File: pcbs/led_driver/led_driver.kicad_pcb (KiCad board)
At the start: 2 copper layers, 21 parts, among them J1 Barrel_Jack, J2 greenLED, J3 Conn_Coaxial, J4 Conn_Coaxial, J5 UVLED, U1 RCD-24, U2 LM350_TO220_9V_output, U3 RCD-24

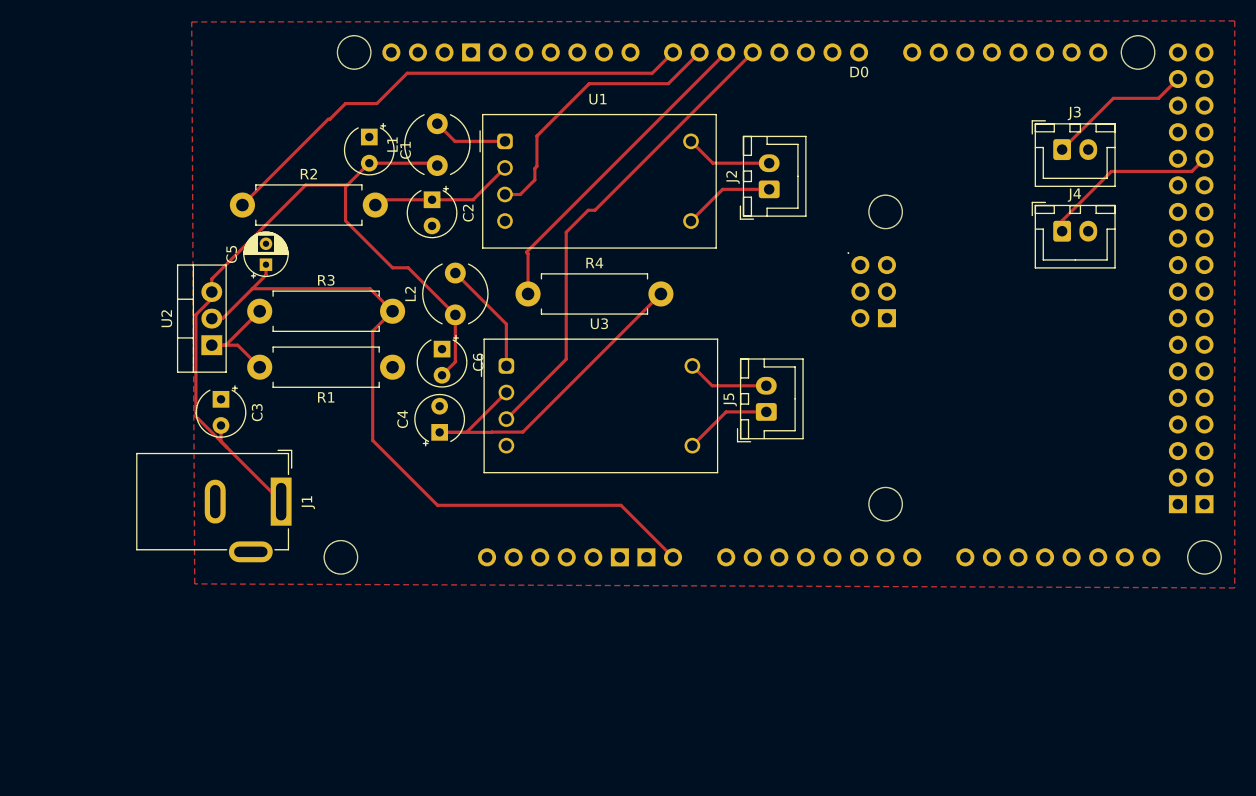
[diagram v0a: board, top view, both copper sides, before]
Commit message: update led der
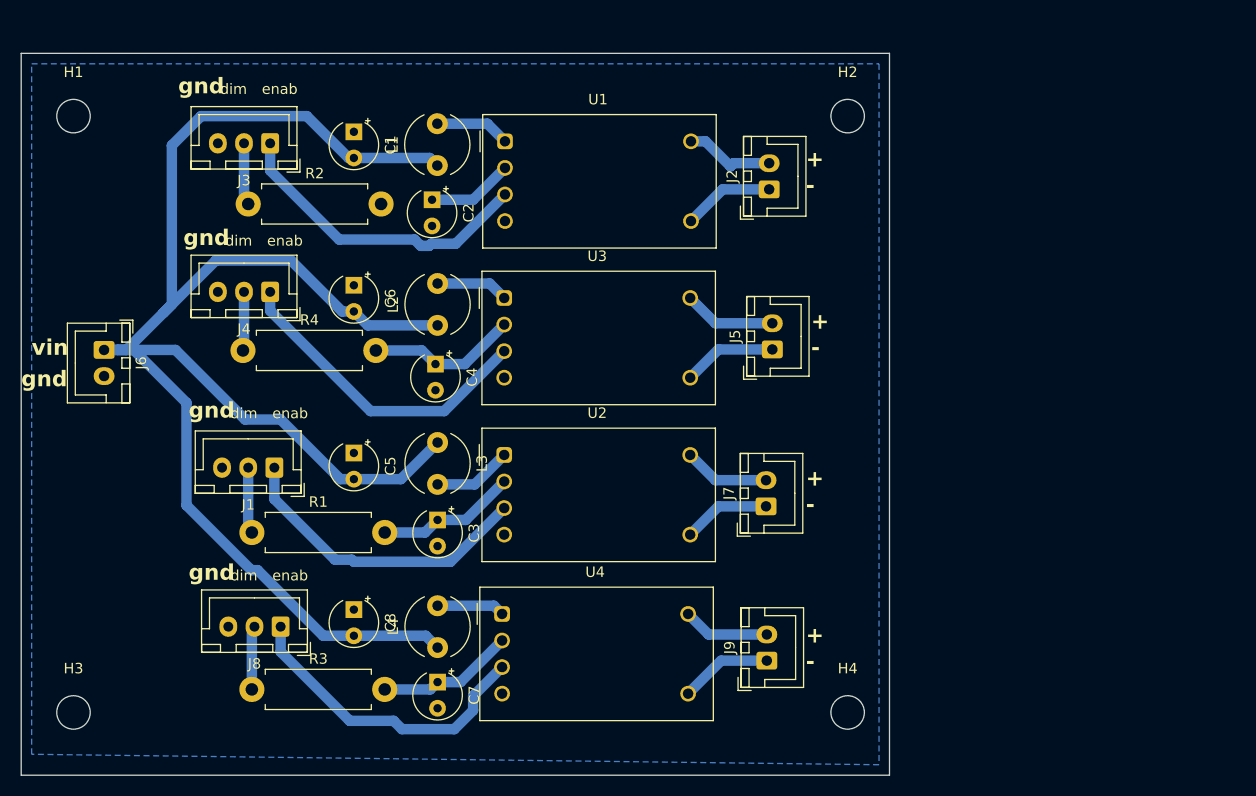
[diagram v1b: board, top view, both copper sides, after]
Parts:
- removed A1: Arduino_Mega2560_R3_Shield, PCM_arduino-library:Arduino_Mega2560_R3_Shield
- added C7: C, Capacitor_THT:CP_Radial_Tantal_D4.5mm_P2.50mm, F.Cu at (111.8, 109.1)
- added C8: 1uF, Capacitor_THT:CP_Radial_Tantal_D4.5mm_P2.50mm, F.Cu at (103.8, 102.2)
- added H1: MountingHole, MountingHole:MountingHole_3.2mm_M3, F.Cu at (77.0, 55.0)
- added H2: MountingHole, MountingHole:MountingHole_3.2mm_M3, F.Cu at (151.0, 55.0)
- added H3: MountingHole, MountingHole:MountingHole_3.2mm_M3, F.Cu at (77.0, 112.0)
- added H4: MountingHole, MountingHole:MountingHole_3.2mm_M3, F.Cu at (151.0, 112.0)
- added J6: power_in, Connector_JST:JST_XH_B2B-XH-A_1x02_P2.50mm_Vertical, F.Cu at (79.9, 77.3)
- added J7: UVLED, Connector_JST:JST_XH_B2B-XH-A_1x02_P2.50mm_Vertical, F.Cu at (143.2, 92.3)
- added J8: Conn_01x03_Pin, Connector_JST:JST_XH_B3B-XH-A_1x03_P2.50mm_Vertical, F.Cu at (96.8, 103.8)
- added J9: UVLED, Connector_JST:JST_XH_B2B-XH-A_1x02_P2.50mm_Vertical, F.Cu at (143.3, 107.0)
- added L3: 22uH, Inductor_THT:L_Radial_D6.0mm_P4.00mm, F.Cu at (111.8, 86.2)
- added L4: 22uH, Inductor_THT:L_Radial_D6.0mm_P4.00mm, F.Cu at (111.8, 105.8)
- added U4: RCD-24, Converter_DCDC:Converter_DCDC_RECOM_RCD-24_THT, F.Cu at (118.0, 102.6)
- C3: value 0.1uF -> C
- C5: footprint Capacitor_THT:CP_Radial_D4.0mm_P2.00mm -> Capacitor_THT:CP_Radial_Tantal_D4.5mm_P2.50mm
- J1: value Barrel_Jack -> Conn_01x03_Pin; footprint Connector_BarrelJack:BarrelJack_GCT_DCJ200-10-A_Horizontal -> Connector_JST:JST_XH_B3B-XH-A_1x03_P2.50mm_Vertical
- J3, J4: value Conn_Coaxial -> Conn_01x03_Pin; footprint Connector_JST:JST_XH_B2B-XH-A_1x02_P2.50mm_Vertical -> Connector_JST:JST_XH_B3B-XH-A_1x03_P2.50mm_Vertical
- R1: value 10k -> R
- R3: value 1.5k -> R
- U2: value LM350_TO220_9V_output -> RCD-24; footprint Package_TO_SOT_THT:TO-220-3_Vertical -> Converter_DCDC:Converter_DCDC_RECOM_RCD-24_THT
- moved J4 75.9 mm to (95.8, 71.8), turned to 180 degrees
- moved J3 75.7 mm to (95.8, 57.6), turned to 180 degrees
- moved R3 36.2 mm to (94.0, 109.8)
- moved U2 29.9 mm to (118.2, 87.4), turned to 0 degrees
- moved R4 27.8 mm to (93.2, 77.4)
- moved C3 23.7 mm to (111.8, 93.6)
- moved R1 20.7 mm to (94.0, 94.8), turned to 0 degrees
- moved C5 19.9 mm to (103.8, 87.2), turned to -90 degrees
- moved C6 10.4 mm to (103.8, 71.2)
- moved C4 6.54 mm to (111.6, 78.7), turned to -90 degrees
- moved U3 6.50 mm to (118.2, 72.4)
- moved J5 6.00 mm to (143.8, 77.3)
- moved J1 3.31 mm to (96.2, 88.6), turned to 180 degrees
- moved L2 1.97 mm to (111.8, 75.0)
- moved C1 1.56 mm to (103.8, 56.5)
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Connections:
- C3 pad 1: GND -> Net-(U2-Analogue_Dimming)
- C3 pad 2: VCC -> GND
- C5 pad 1: Net-(U2-VO) -> GND
- C5 pad 2: GND -> VCC
- J1 pad 1: VCC -> Net-(J1-Pin_1)
- J1 pad 2: GND -> Net-(J1-Pin_2)
- J1 pad 3: (no net) -> GND
- J3 pad 1: Net-(J3-In) -> Net-(J3-Pin_1)
- J3 pad 2: GND -> Net-(J3-Pin_2)
- J4 pad 1: Net-(J4-In) -> Net-(J4-Pin_1)
- J4 pad 2: GND -> Net-(J4-Pin_2)
- R1 pad 1: GND -> Net-(J1-Pin_2)
- R1 pad 2: Net-(U2-ADJ) -> Net-(U2-Analogue_Dimming)
- R2 pad 1: analogue1 -> Net-(J3-Pin_2)
- R3 pad 1: Net-(U2-ADJ) -> Net-(J8-Pin_2)
- R3 pad 2: Net-(U2-VO) -> Net-(U4-Analogue_Dimming)
- R4 pad 1: analogue2 -> Net-(J4-Pin_2)
- U1 pad 3: PWM1 -> Net-(J3-Pin_1)
- U2 pad 1: Net-(U2-ADJ) -> Net-(U2-+Vin)
- U2 pad 2: Net-(U2-VO) -> Net-(U2-Analogue_Dimming)
- U2 pad 3: VCC -> Net-(J1-Pin_1)
- U3 pad 3: PWM2 -> Net-(J4-Pin_1)
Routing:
- net VCC: track 79.2 -> 169.4 mm
- net Net-(U2-VO): track 68.7 -> 0.00 mm
- net analogue1: track 47.2 -> 0.00 mm
- net PWM2: track 45.2 -> 0.00 mm
- net analogue2: track 31.1 -> 0.00 mm
- net Net-(J4-Pin_1): track 0.00 -> 30.5 mm
- net Net-(J3-Pin_1): track 0.00 -> 30.1 mm
- net Net-(J8-Pin_1): track 0.00 -> 29.9 mm
- net Net-(J1-Pin_1): track 0.00 -> 29.6 mm
- net PWM1: track 26.6 -> 0.00 mm
- net Net-(U3-Analogue_Dimming): track 34.6 -> 14.4 mm
- net Net-(J4-In): track 17.1 -> 0.00 mm
- net Net-(J3-In): track 13.9 -> 0.00 mm
- net Net-(U2-Analogue_Dimming): track 0.00 -> 13.4 mm
- net Net-(U4-Analogue_Dimming): track 0.00 -> 13.2 mm
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- added copper zone on B.Cu, net GND
- removed copper zone on F.Cu, net GND
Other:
- board outline added: 83 x 69 mm
- board text added: "+"
- board text added: "-"
- board text added: "dim"
- board text added: "enab"
- board text added: "gnd"
- board text added: "vin"
